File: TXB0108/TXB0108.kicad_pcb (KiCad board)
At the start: 2 copper layers, 15.2 x 25.4 mm, 10 parts, among them J1 Conn_01x10, J2 Conn_01x10

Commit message: Silkscreen Edits
Dimensions moved to Drawings Layer
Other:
- rule pad_to_mask_clearance: 0.051 -> 0
- rule solder_mask_min_width: 0.25 -> 0.1
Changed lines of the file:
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@@
     (pad_size 1.7 1.7)
     (pad_drill 1)
-    (pad_to_mask_clearance 0.051)
-    (solder_mask_min_width 0.25)
+    (pad_to_mask_clearance 0)
+    (solder_mask_min_width 0.1)
     (aux_axis_origin 0 0)
     (visible_elements 7FFFFFFF)
     (pcbplotparams
-      (layerselection 0x010fc_ffffffff)
+      (layerselection 0x010f0_ffffffff)
       (usegerberextensions false)
       (usegerberattributes false)
@@
       (viasonmask false)
       (mode 1)
-      (useauxorigin false)
+      (useauxorigin true)
       (hpglpennumber 1)
       (hpglpenspeed 20)
@@
       (psa4output false)
       (plotreference true)
-      (plotvalue true)
+      (plotvalue false)
       (plotinvisibletext false)
       (padsonsilk false)
@@
       (outputformat 1)
       (mirror false)
-      (drillshape 1)
+      (drillshape 0)
       (scaleselection 1)
-      (outputdirectory ""))
+      (outputdirectory "../../Gerbers/TXB0108/"))
   )
   (net 0 "")
@@
     )
   )
-  (dimension 22.86 (width 0.12) (layer F.SilkS)
-    (gr_text "22.860 mm" (at 149.86 115.57 270) (layer F.SilkS)
+  (dimension 22.86 (width 0.12) (layer Dwgs.User)
+    (gr_text "22.860 mm" (at 149.86 115.57 270) (layer Dwgs.User)
       (effects (font (size 1 1) (thickness 0.15)) hide)
     )
@@
     (arrow2b (pts (xy 148.59 104.14) (xy 149.176421 105.266504)))
   )
-  (dimension 25.4 (width 0.12) (layer F.SilkS)
-    (gr_text "25.400 mm" (at 152.654 115.57 270) (layer F.SilkS)
+  (dimension 25.4 (width 0.12) (layer Dwgs.User)
+    (gr_text "25.400 mm" (at 152.654 115.57 270) (layer Dwgs.User)
       (effects (font (size 1 1) (thickness 0.15)) hide)
     )
@@
     (arrow2b (pts (xy 151.384 102.87) (xy 151.970421 103.996504)))
   )
-  (dimension 12.7 (width 0.12) (layer F.SilkS)
-    (gr_text "12.700 mm" (at 138.43 99.822) (layer F.SilkS)
+  (dimension 12.7 (width 0.12) (layer Dwgs.User)
+    (gr_text "12.700 mm" (at 138.43 99.822) (layer Dwgs.User)
       (effects (font (size 1 1) (thickness 0.15)) hide)
     )
@@
     (arrow2b (pts (xy 132.08 101.092) (xy 133.206504 100.505579)))
   )
-  (dimension 15.24 (width 0.12) (layer F.SilkS)
-    (gr_text "15.240 mm" (at 138.43 97.409) (layer F.SilkS)
+  (dimension 15.24 (width 0.12) (layer Dwgs.User)
+    (gr_text "15.240 mm" (at 138.43 97.409) (layer Dwgs.User)
       (effects (font (size 1 1) (thickness 0.15)) hide)
     )

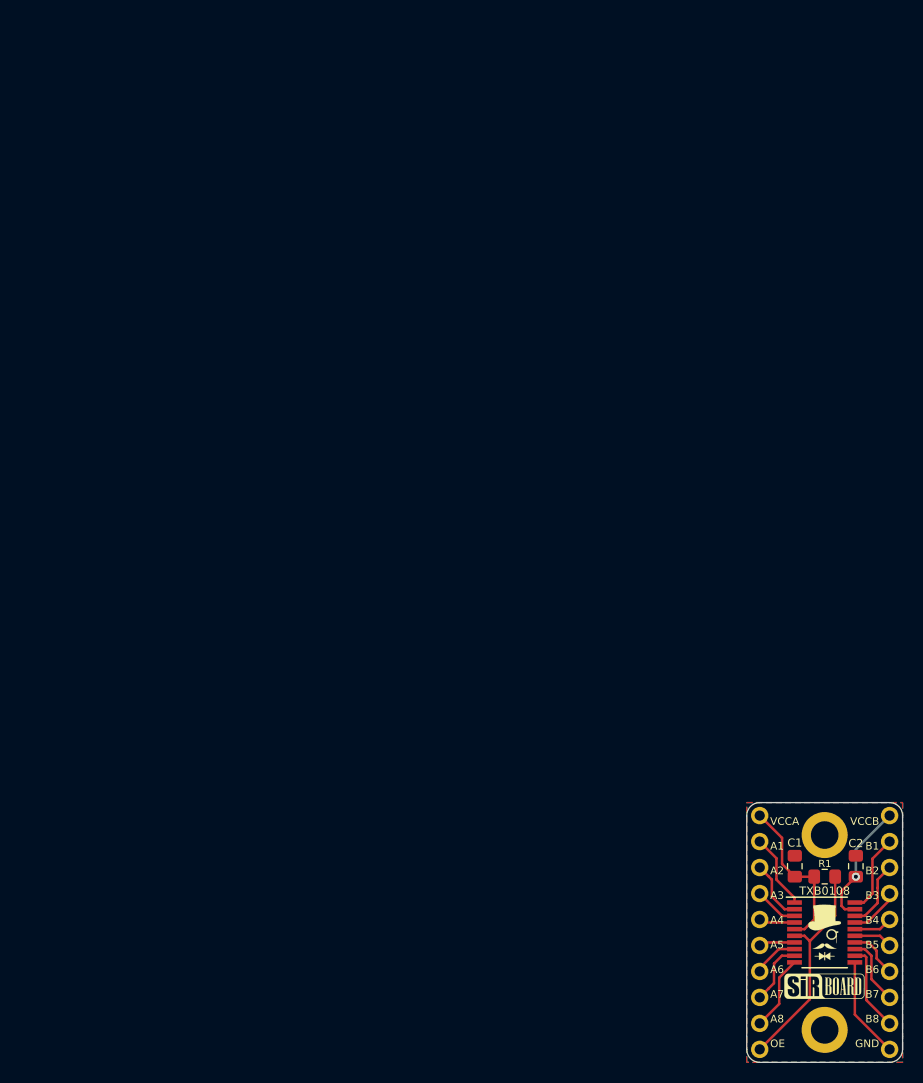
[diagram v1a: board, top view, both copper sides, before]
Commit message: Part Numbers Added
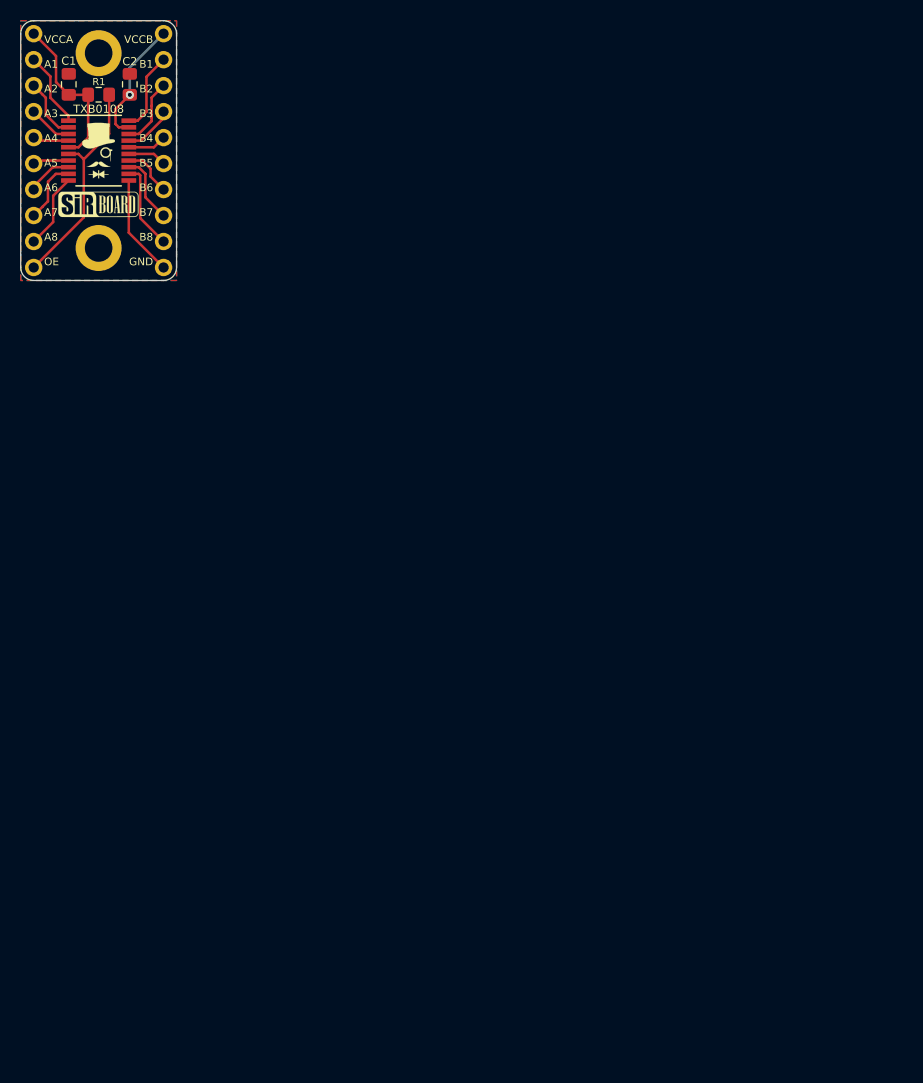
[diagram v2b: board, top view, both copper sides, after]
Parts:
- moved C2 104.3 mm to (70.5, 32.6)
- moved G*** 104.3 mm to (67.4, 39.1)
- moved J1 104.3 mm to (61.1, 27.7)
- moved J2 104.3 mm to (73.8, 27.7)
- moved R1 104.3 mm to (67.4, 33.7)
- moved REF** 104.3 mm to (67.4, 48.6)
- moved REF** 104.3 mm to (67.4, 29.6)
- moved TXB0108 104.3 mm to (67.4, 39.1)
- moved C1 104.3 mm to (64.5, 32.6)
- moved G*** 104.3 mm to (67.4, 44.4)
